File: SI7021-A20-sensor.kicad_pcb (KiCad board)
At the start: 2 copper layers, 20.1 x 15.7 mm, 16 parts, among them J1 Conn_01x05, Q1 BSS138, Q2 BSS138, U1 Si7021-A20, U2 MIC5225-3.3

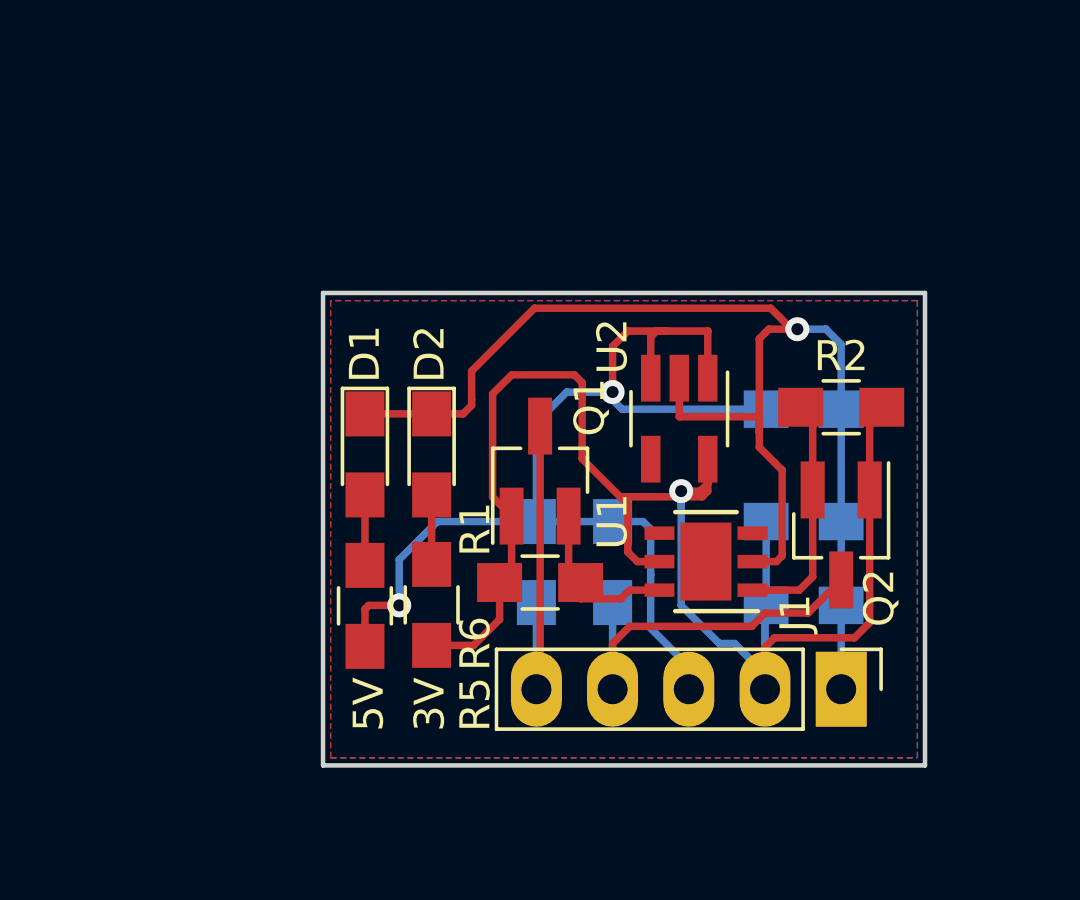
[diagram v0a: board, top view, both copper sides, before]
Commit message: update,
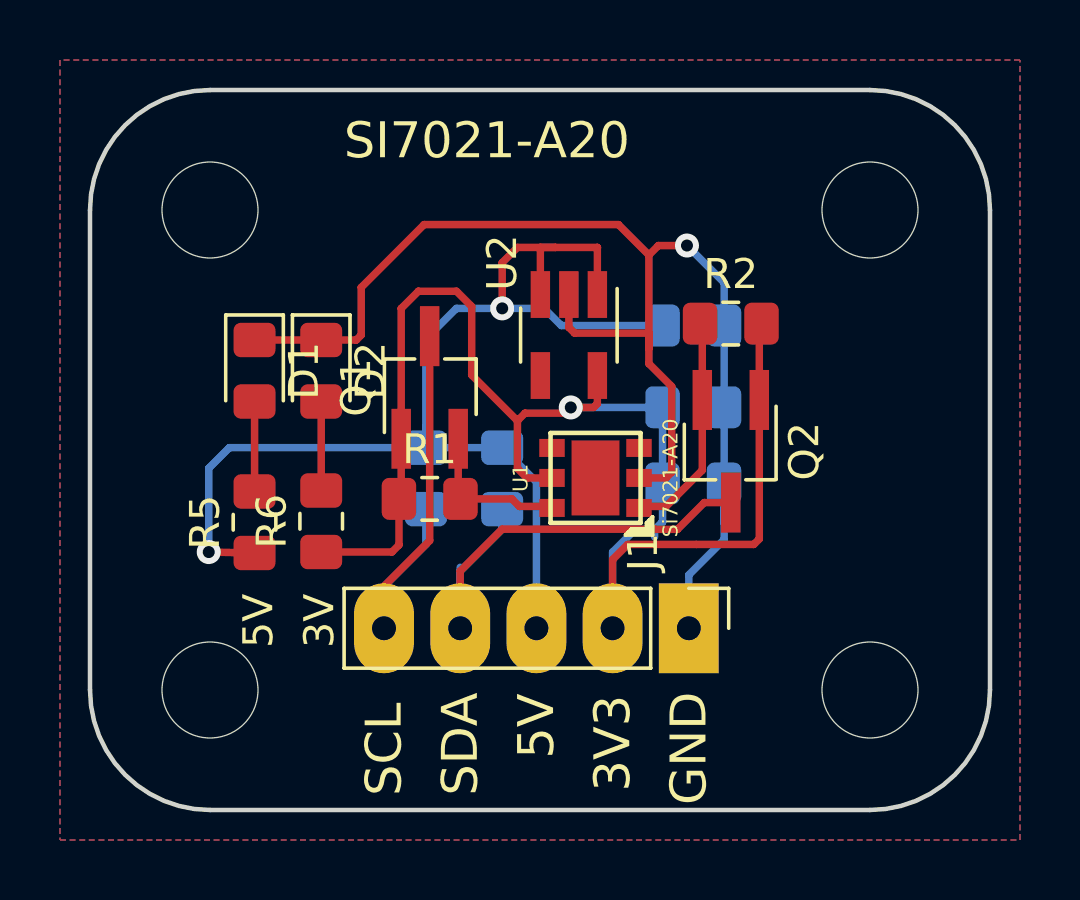
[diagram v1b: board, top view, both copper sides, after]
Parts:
- added REF**: MountingHole_3.2mm_M3, MountingHole:MountingHole_3.2mm_M3, F.Cu at (45.0, 30.0)
- added REF**: MountingHole_3.2mm_M3, MountingHole:MountingHole_3.2mm_M3, F.Cu at (67.0, 30.0)
- added REF**: MountingHole_3.2mm_M3, MountingHole:MountingHole_3.2mm_M3, F.Cu at (45.0, 46.0)
- added REF**: MountingHole_3.2mm_M3, MountingHole:MountingHole_3.2mm_M3, F.Cu at (67.0, 46.0)
- C1, C2, C3: footprint Capacitors_SMD:C_0805_HandSoldering -> Capacitor_SMD:C_0805_2012Metric_Pad1.15x1.40mm_HandSolder
- D1, D2: footprint LEDs:LED_0805_HandSoldering -> LED_SMD:LED_0805_2012Metric_Pad1.15x1.40mm_HandSolder
- J1: footprint footprint-lib:Pin_Header_Straight_1x05_Pitch2.54mm -> footprint-lib.pretty:Pin_Header_Straight_1x05_Pitch2.54mm
- Q1, Q2: footprint TO_SOT_Packages_SMD:SOT-23_Handsoldering -> Package_TO_SOT_SMD:TSOT-23_HandSoldering
- R1, R2, R3, R4, R5, R6: footprint Resistors_SMD:R_0805_HandSoldering -> Resistor_SMD:R_0805_2012Metric_Pad1.15x1.40mm_HandSolder
- U1: footprint footprint-lib:DFN-6-1EP_3x3mm_Pitch0.95mm -> w_smd_qfn:dfn6-3x3
- U2: footprint TO_SOT_Packages_SMD:SOT-23-5_HandSoldering -> Package_TO_SOT_SMD:SOT-23-5_HandSoldering
- moved C1 5.48 mm to (61.1, 39.1)
- moved J1 5.47 mm to (61.0, 43.9)
- moved C3 5.30 mm to (61.1, 36.6)
- moved C2 4.62 mm to (61.1, 33.9)
- moved Q2 4.62 mm to (62.4, 38.0)
- moved R2 4.62 mm to (62.4, 33.8)
- moved D1 4.62 mm to (46.5, 35.4)
- moved D2 4.62 mm to (48.7, 35.4)
- moved Q1 4.62 mm to (52.3, 35.9)
- moved R1 4.62 mm to (52.3, 39.6)
- moved R3 4.62 mm to (52.2, 38.9)
- moved R4 4.62 mm to (54.7, 38.9)
- moved R5 4.62 mm to (46.5, 40.4)
- moved R6 4.62 mm to (48.7, 40.4)
- moved U1 4.62 mm to (57.9, 38.9), turned to 90 degrees
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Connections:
- U2 pad 4: (no net) -> Net-(U2-Pad4)
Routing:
- net /SDA: track 13.6 -> 18.5 mm
- net +5V: track 39.0 -> 42.2 mm
- net +3V3: track 54.0 -> 51.6 mm
- net /SCL: track 12.5 -> 14.4 mm
- net GND: track 45.1 -> 45.6 mm
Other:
- board size 20.1 x 15.7 mm -> 30 x 24 mm
- board text added: "3V3"
- board text added: "GND"
- board text added: "SCL"
- board text added: "SDA"
- board text added: "SI7021-A20"
- board text removed: "SCL SDA +5V +3V3 GND"

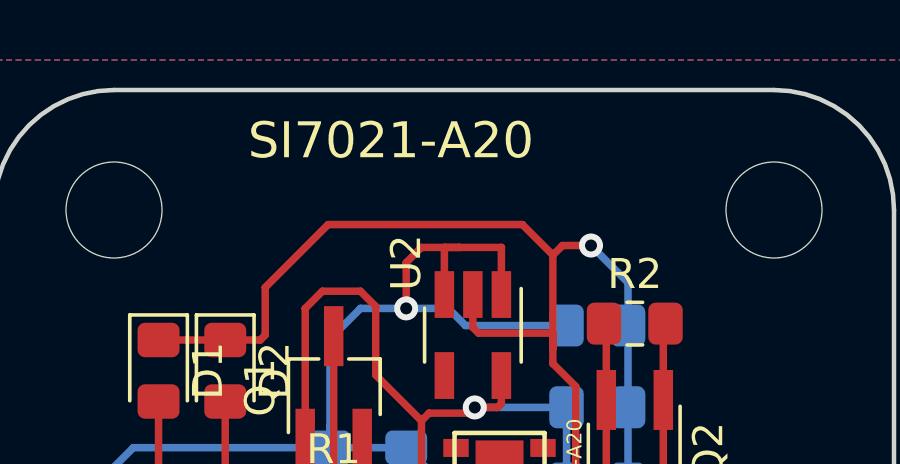
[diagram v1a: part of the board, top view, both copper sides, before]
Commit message: update
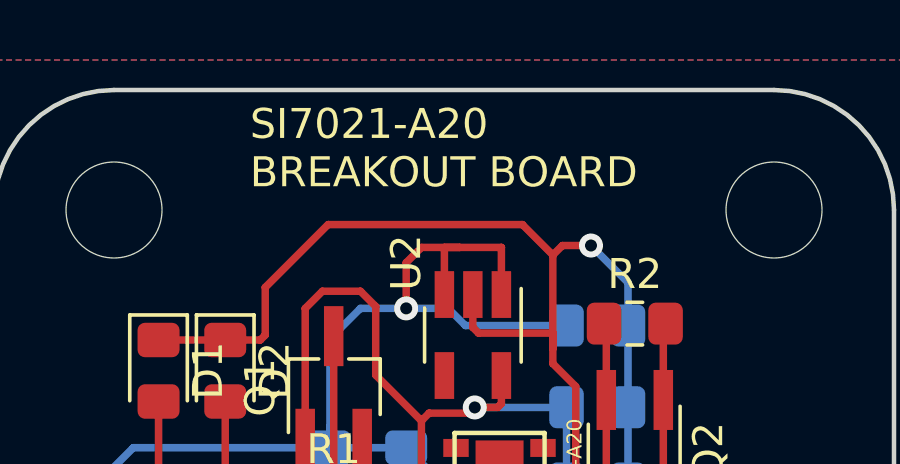
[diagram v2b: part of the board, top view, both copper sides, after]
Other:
- board text added: "SI7021-A20 BREAKOUT BOARD"
- board text removed: "SI7021-A20"
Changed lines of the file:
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@@
     (pad 1 np_thru_hole circle (at 0 0) (size 3.2 3.2) (drill 3.2) (layers *.Cu *.Mask))
   )
-  (gr_text SI7021-A20 (at 54.229 27.686) (layer F.SilkS)
-    (effects (font (size 1.2 1.2) (thickness 0.2)))
+  (gr_text "SI7021-A20\nBREAKOUT BOARD" (at 49.53 27.94) (layer F.SilkS)
+    (effects (font (size 1 1) (thickness 0.2)) (justify left))
   )
   (gr_text GND (at 60.96 47.944286 90) (layer F.SilkS)
